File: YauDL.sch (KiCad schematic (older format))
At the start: 40 parts, among them K1 HEATSINK, Q1 IRL3803, Q2 IRL3803, Q3 AO3401, Q4 AO3401, SW1 SWITCH_INV, T1 Binding post, T2 Binding post, T3 Binding post, T4 Binding post, U1 TS2940, U2 LM2904, U3 TCM829

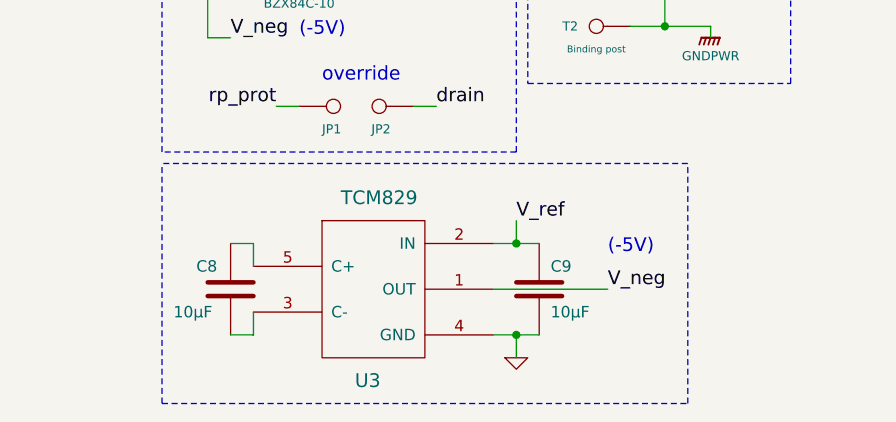
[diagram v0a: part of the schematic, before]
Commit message: Tweaks...
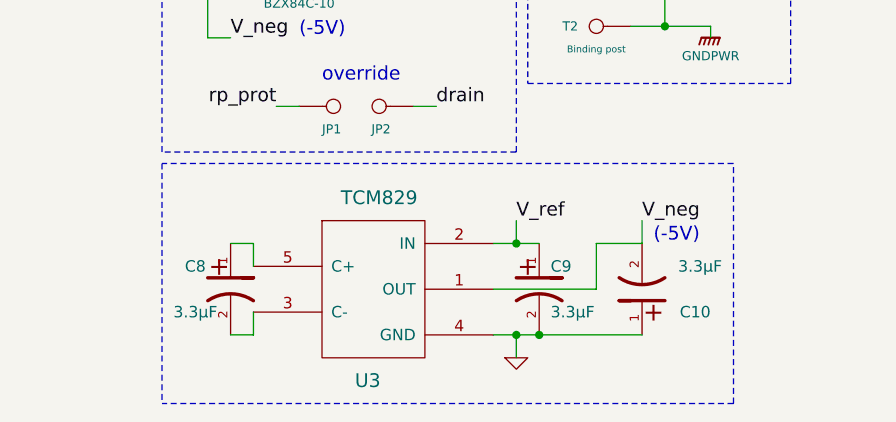
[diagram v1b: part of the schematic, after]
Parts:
- removed C8, C9: 10µF, symbol C
- added C10, C8, C9: 3.3µF, symbol CP1
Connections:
- net GND: now also C10.1, C9.2
- net V_neg: now also C10.2
- net V_ref: now also C9.1
- net at U3.3 (C-): now also C8.2
- net at U3.5 (C+): now also C8.1
